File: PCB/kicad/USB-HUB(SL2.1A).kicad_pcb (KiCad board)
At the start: 2 copper layers, 50 x 20 mm, 33 parts, among them U1 SL2.1S

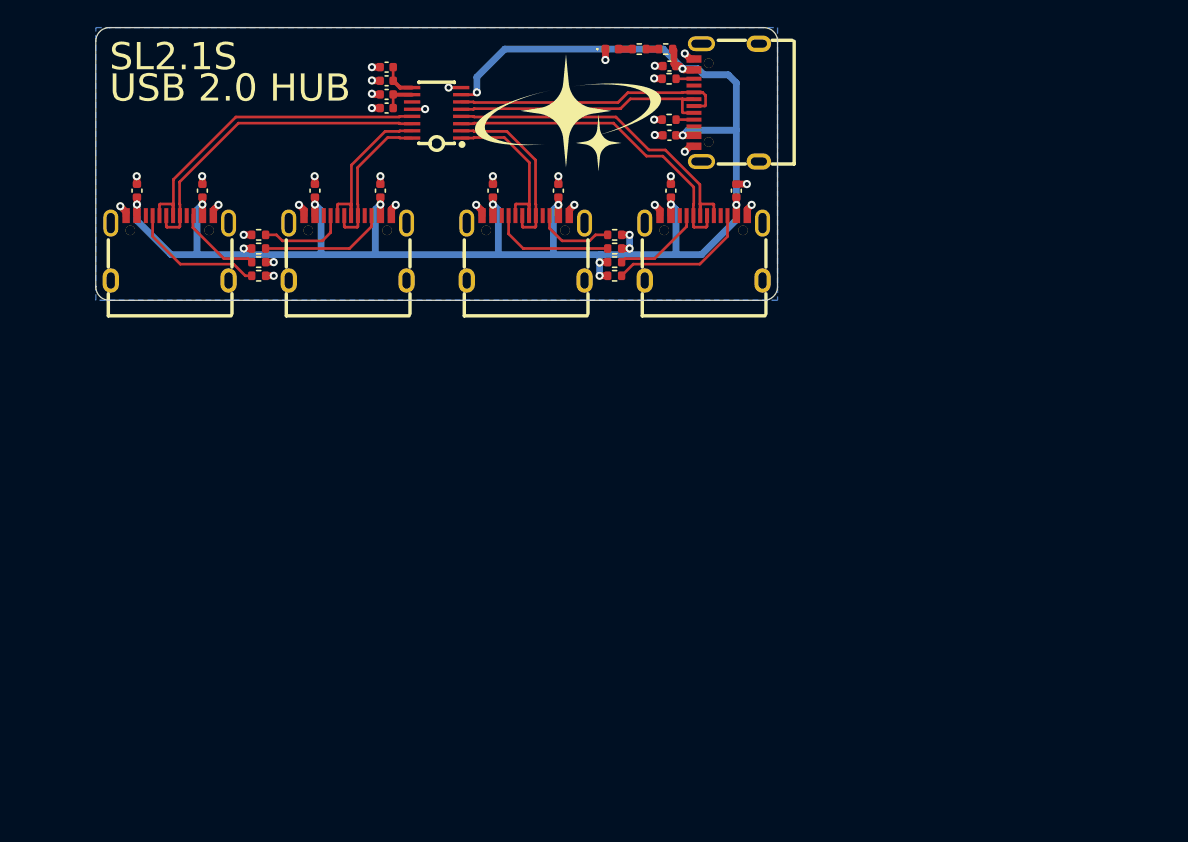
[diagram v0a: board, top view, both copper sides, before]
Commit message: rev 2.0
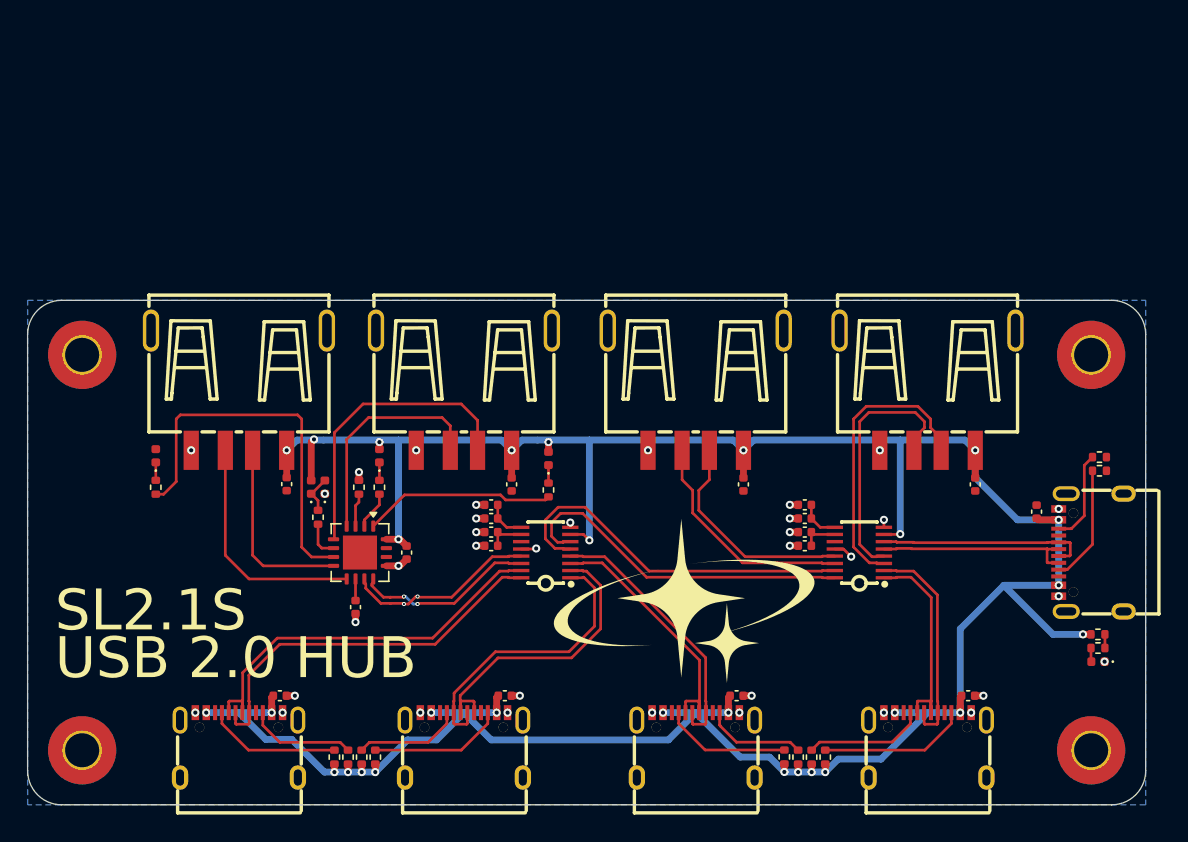
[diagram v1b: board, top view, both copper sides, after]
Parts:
- removed C9: 100nF, Capacitor_SMD:C_0402_1005Metric
- added C15: 10uF, Capacitor_SMD:C_0402_1005Metric, F.Cu at (148.0, 65.0)
- added C16: 100nF, Capacitor_SMD:C_0402_1005Metric, F.Cu at (148.0, 66.0)
- added C17: 10uF, Capacitor_SMD:C_0402_1005Metric, F.Cu at (148.0, 68.0)
- added C18: 100nF, Capacitor_SMD:C_0402_1005Metric, F.Cu at (148.0, 67.0)
- added C19: 1uF, Capacitor_SMD:C_0402_1005Metric, F.Cu at (138.1, 72.5)
- added C20: 1uF, Capacitor_SMD:C_0402_1005Metric, F.Cu at (141.8, 68.5)
- added D2: LED, LED_SMD:LED_0402_1005Metric, F.Cu at (152.2, 61.6)
- added D3: LED, LED_SMD:LED_0402_1005Metric, F.Cu at (139.8, 61.4)
- added D4: LED, LED_SMD:LED_0402_1005Metric, F.Cu at (123.4, 61.4)
- added D5: LED, LED_SMD:LED_0402_1005Metric, F.Cu at (134.8, 63.7)
- added D6: LED, LED_SMD:LED_0402_1005Metric, F.Cu at (135.8, 63.7)
- added H1: MountingHole_Pad_MP, MountingHole:MountingHole_2.5mm_Pad_TopBottom, F.Cu at (192.0, 54.0)
- added H2: MountingHole_Pad_MP, MountingHole:MountingHole_2.5mm_Pad_TopBottom, F.Cu at (192.0, 83.0)
- added H3: MountingHole_Pad_MP, MountingHole:MountingHole_2.5mm_Pad_TopBottom, F.Cu at (118.0, 54.0)
- added H4: MountingHole_Pad_MP, MountingHole:MountingHole_2.5mm_Pad_TopBottom, F.Cu at (118.0, 83.0)
- added J1: USB_A, easyeda2kicad:USB-A-TH_10.0QHHTZB6.3, F.Cu at (146.0, 56.6)
- added J2: USB_A, easyeda2kicad:USB-A-TH_10.0QHHTZB6.3, F.Cu at (129.5, 56.6)
- added J3: USB_A, easyeda2kicad:USB-A-TH_10.0QHHTZB6.3, F.Cu at (180.0, 56.6)
- added J4: USB_A, easyeda2kicad:USB-A-TH_10.0QHHTZB6.3, F.Cu at (163.0, 56.6)
- added R13: 5.1K, Resistor_SMD:R_0402_1005Metric, F.Cu at (152.2, 63.9)
- added R14: 5.1K, Resistor_SMD:R_0402_1005Metric, F.Cu at (139.8, 63.7)
- added R15: 5.1K, Resistor_SMD:R_0402_1005Metric, F.Cu at (123.4, 63.7)
- added R16: 5.1K, Resistor_SMD:R_0402_1005Metric, F.Cu at (135.3, 65.9)
- added SW1: SW_Push_45deg, Resistor_SMD:R_0402_1005Metric, F.Cu at (138.3, 63.7)
- added U2: SL2.1S, easyeda2kicad:SSOP-16_L4.6-W2.6-P0.53-LS4.0-BL, F.Cu at (152.0, 68.5)
- added U3: MCP2221AxML, Package_DFN_QFN:QFN-16-1EP_4x4mm_P0.65mm_EP2.5x2.5mm, F.Cu at (138.4, 68.5)
- C5, C6, C7, C8: value 100nF -> 1uF
- moved C11 65.6 mm to (188.0, 65.5)
- moved D1 57.3 mm to (192.5, 76.5), turned to 180 degrees
- moved R12 55.3 mm to (192.5, 75.5)
- moved R10 53.7 mm to (170.5, 83.5), turned to -90 degrees
- moved R11 53.4 mm to (192.5, 74.5), turned to 0 degrees
- moved USB5 53.1 mm to (163.0, 82.6)
- moved R9 52.3 mm to (169.5, 83.5), turned to -90 degrees
- moved C6 49.4 mm to (166.5, 63.5), turned to -90 degrees
- moved C13 46.4 mm to (166.0, 79.0), turned to 0 degrees
- moved U1 44.7 mm to (175.0, 68.5)
- moved C1 44.4 mm to (171.0, 65.0)
- moved C2 44.4 mm to (171.0, 66.0)
- moved C3 44.4 mm to (171.0, 68.0)
- moved C4 44.4 mm to (171.0, 67.0)
- moved R6 43.0 mm to (137.5, 83.5), turned to -90 degrees
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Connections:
- USB2 pad 5: /D1- -> /D2-
- USB2 pad 6: /D1+ -> /D2+
- USB2 pad 7: /D1- -> /D2-
- USB2 pad 8: /D1+ -> /D2+
- USB3 pad 5: /D2- -> /D7-
- USB3 pad 6: /D2+ -> /D7+
- USB3 pad 7: /D2- -> /D7-
- USB3 pad 8: /D2+ -> /D7+
- USB4 pad 5: /D3- -> /D6-
- USB4 pad 6: /D3+ -> /D6+
- USB4 pad 7: /D3- -> /D6-
- USB4 pad 8: /D3+ -> /D6+
- USB5 pad 5: /D4- -> /D5-
- USB5 pad 6: /D4+ -> /D5+
- USB5 pad 7: /D4- -> /D5-
- USB5 pad 8: /D4+ -> /D5+
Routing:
- net VBUS: track 130.3 -> 217.7 mm, vias 19 -> 29
- net /D7-: track 0.00 -> 29.1 mm
- net /D7+: track 0.00 -> 28.4 mm
- net /LED_I2C: track 0.00 -> 28.0 mm
- net /D6+: track 0.00 -> 22.1 mm
- net /UTX: track 0.00 -> 21.9 mm
- net /D6-: track 0.00 -> 21.3 mm
- net /D5+: track 0.00 -> 19.7 mm
- net /D5-: track 0.00 -> 19.0 mm
- net /SCL: track 0.00 -> 17.3 mm
- net /URX: track 0.00 -> 16.7 mm
- net /D3-: track 11.9 -> 27.1 mm
- net /D3+: track 11.1 -> 25.6 mm
- net /D8-: track 0.00 -> 14.1 mm, vias 0 -> 2
- net /LED_URX: track 0.00 -> 14.0 mm
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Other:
- board size 50 x 20 mm -> 82 x 37 mm
